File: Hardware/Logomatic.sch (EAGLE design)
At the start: 63 parts, among them Q1 12MHz, Q2 32kHz, Q4 TRANSISTOR_PNPSMD, U1 MCP73831, U2 3.3V, U3 USD-SOCKETNEW, U4 LPC213X, X1 USBSMD

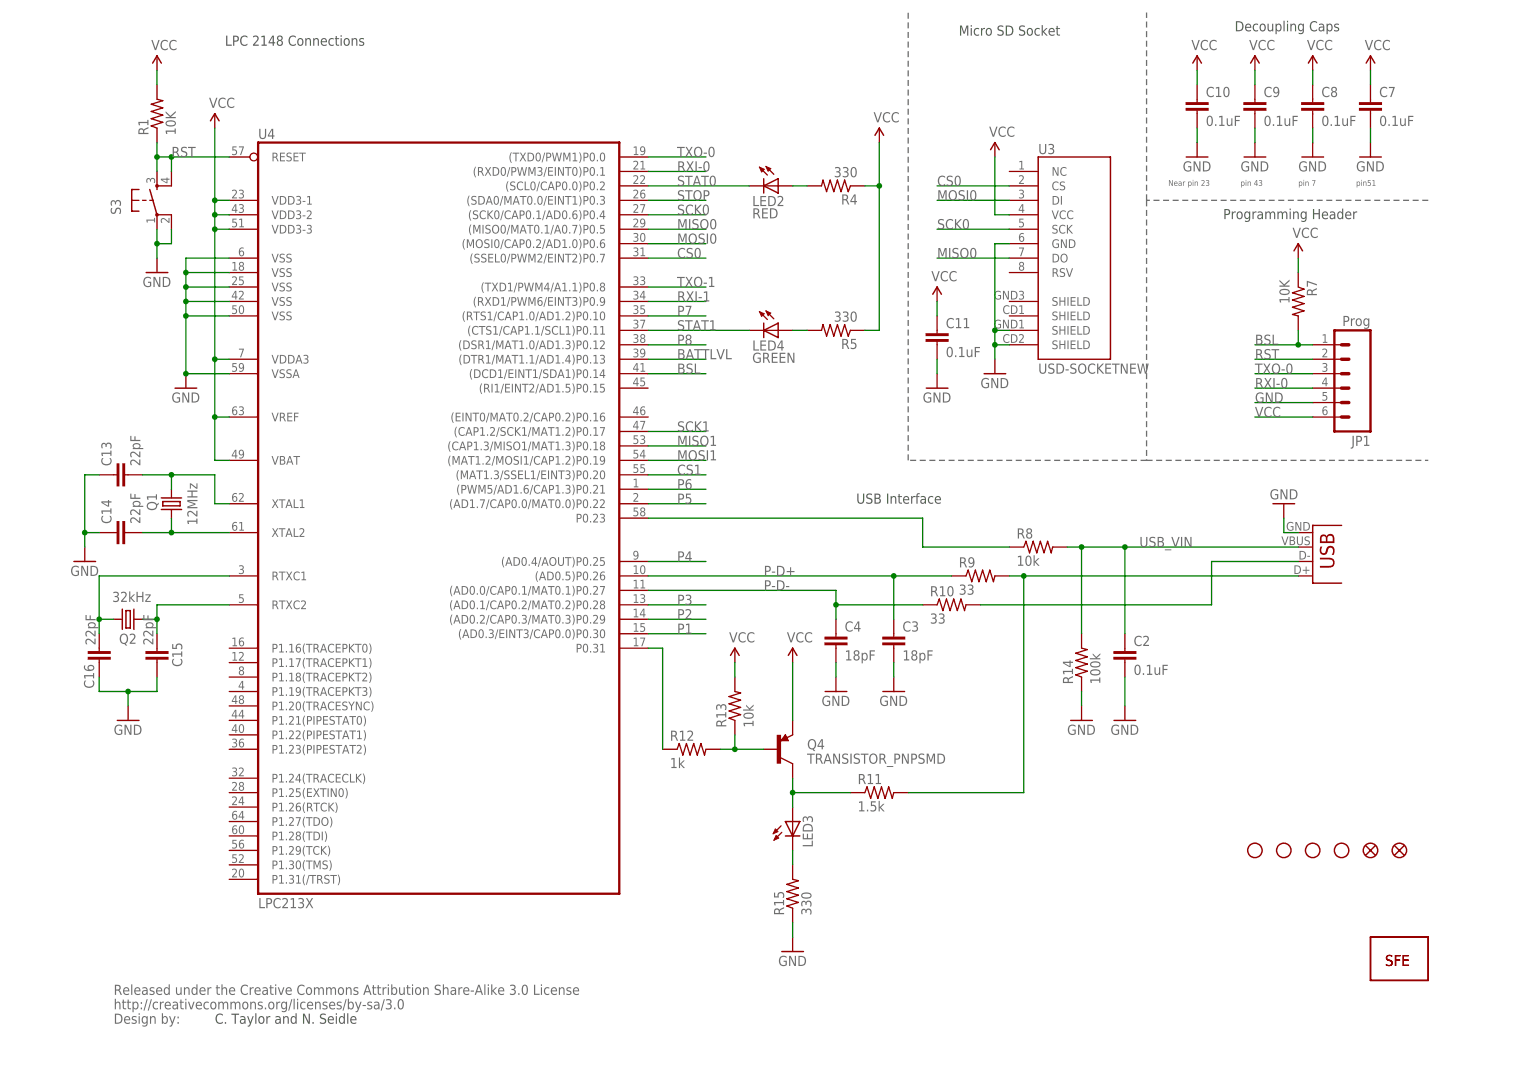
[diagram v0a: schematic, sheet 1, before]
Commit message: Version 2.7 board commit
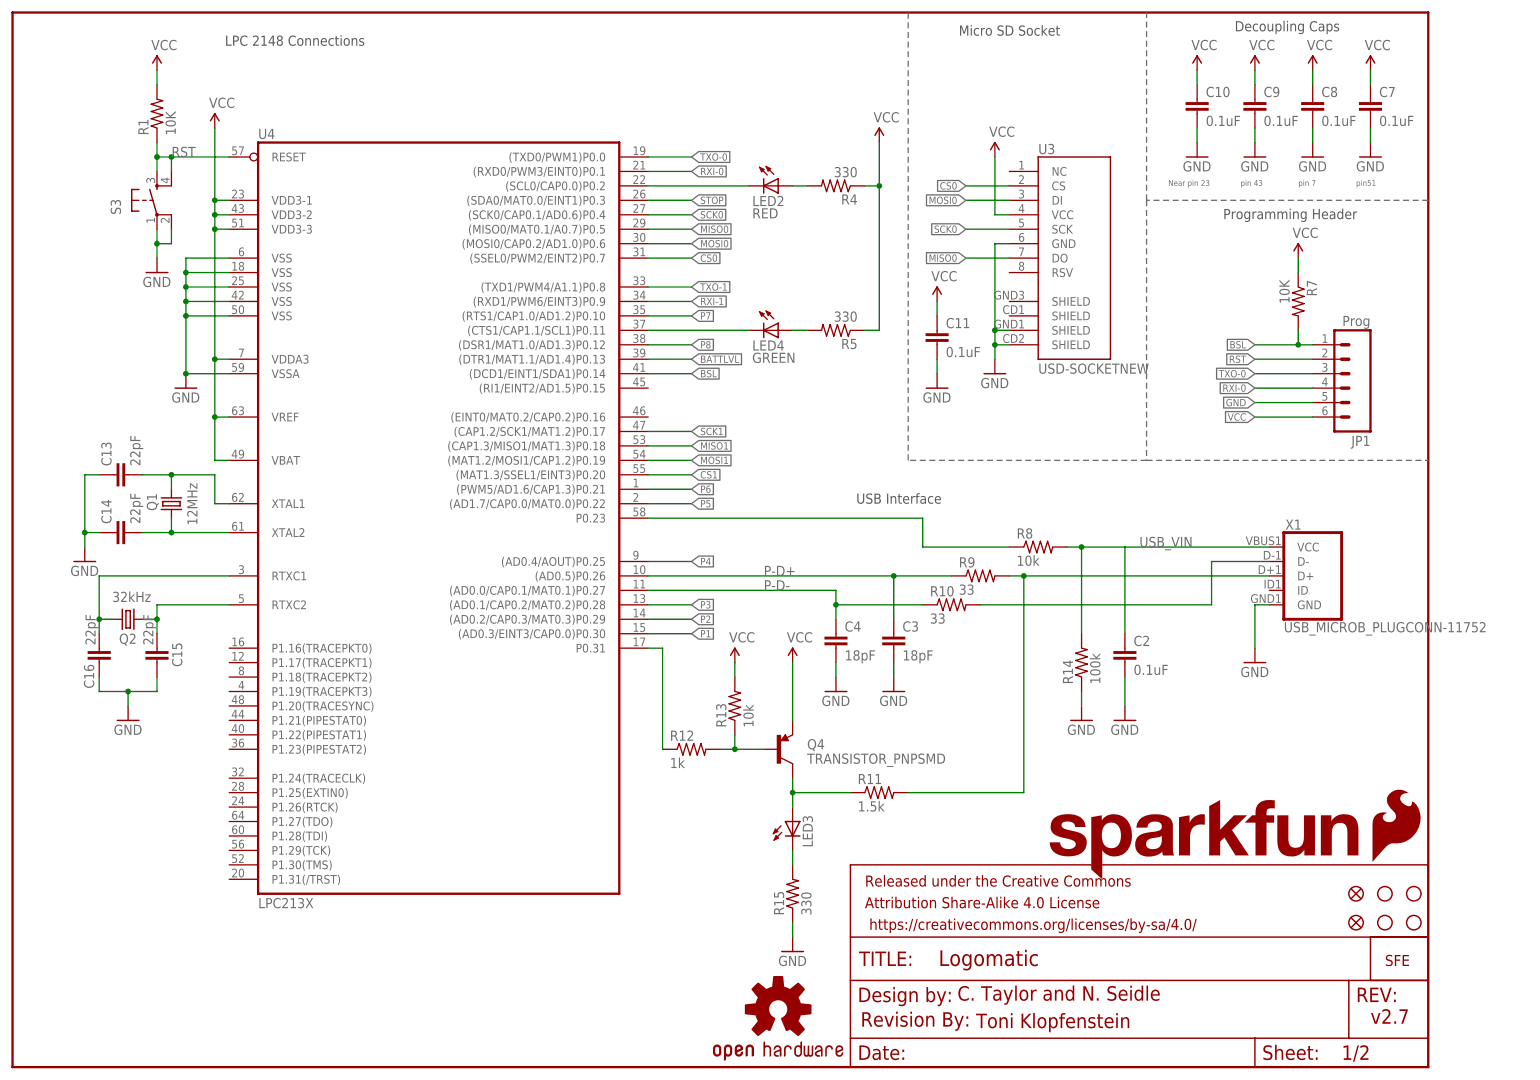
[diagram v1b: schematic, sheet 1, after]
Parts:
- removed U$9: CREATIVE_COMMONS, SparkFun:CREATIVE_COMMONS
- added FRAME2, FRAME4: FRAME-LETTER, SparkFun-Aesthetics:FRAME-LETTER
- added LOGO1: OSHW-LOGOL, SparkFun-Aesthetics:OSHW-LOGOL
- added LOGO2: SFE_LOGO_NAME.1_INCH, SparkFun-Aesthetics:SFE_LOGO_NAME.1_INCH
- added U$10: REVISION, SparkFun-Aesthetics:REVISION
- C1, C10, C11, C12, C2, C7, C8, C9: device SparkFunEagle-6-6-07:CAP0402 -> SparkFun-Capacitors:0.1UF-25V(+80/-20%)(0603)
- C13, C14, C15, C16: device SparkFunEagle-6-6-07:CAP0402 -> SparkFun-Capacitors:22PF-50V-5%(0603)
- C17, C5: device SparkFun:CAP0402-CAP -> SparkFun-Capacitors:4.7UF-6.3V-10%(0603)0603
- C3, C4: device SparkFunEagle-6-6-07:CAP0402 -> SparkFun-Capacitors:18PF-50V-5%(0603)
- C6: device SparkFun:CAP_POL1206 -> SparkFun-Capacitors:10UF-16V-10%(TANT)
- R1, R13, R6, R7, R8: device SparkFunEagle-6-6-07:RESISTOR0402 -> SparkFun-Resistors:10KOHM1/10W1%(0603)0603
- R10, R9: device SparkFunEagle-6-6-07:RESISTOR0402 -> SparkFun-Resistors:33OHM1/10W1%(0603)
- R11: device SparkFunEagle-6-6-07:RESISTOR0402 -> SparkFun-Resistors:1.5KOHM1/10W1%(0603)
- R12: device SparkFunEagle-6-6-07:RESISTOR0402 -> SparkFun-Resistors:1KOHM1/10W1%(0603)
- R14: device SparkFunEagle-6-6-07:RESISTOR0402 -> SparkFun-Resistors:100KOHM1/10W1%(0603)
- R15, R4, R5: device SparkFunEagle-6-6-07:RESISTOR0402 -> SparkFun-Resistors:330OHM1/10W1%(0603)
- R16, R17: device SparkFun:RESISTOR0402-RES -> SparkFun-Resistors:1MOHM1/10W1%(0603)
- R2: device SparkFun:RESISTOR0402-RES -> SparkFun-Resistors:2.0KOHM1/10W5%(0603)
- R3: device SparkFun:RESISTOR0402-RES -> SparkFun-Resistors:330OHM1/10W1%(0603)
- U$6: value LOGO-SFENEW -> SFE_LOGO_FLAME1_INCH; device SparkFun:LOGO-SFENEW -> SparkFun-Aesthetics:SFE_LOGO_FLAME1_INCH
- U3: device SparkFun:USD-SOCKETNEW -> SparkFun-Connectors:USD-SOCKETNEW
- X1: value USBSMD -> USB_MICROB_PLUGCONN-11752; device SparkFun:USBSMD -> SparkFun-Connectors:USB_MICROB_PLUGCONN-11752
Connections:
- net USB_VIN: now also X1.VCC; no longer X1.VBUS
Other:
- note added: "Toni Klopfenstein"
- note added: "v2.7"
